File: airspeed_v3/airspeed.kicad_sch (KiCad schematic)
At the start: 27 parts, among them J1 Header, J2 GPS, J3 GPS, J4 ScreenIO, U1 XGZP6897D, U3 SHT4x, U5 XGZP6897D, U6 BME280, U8 BMP280

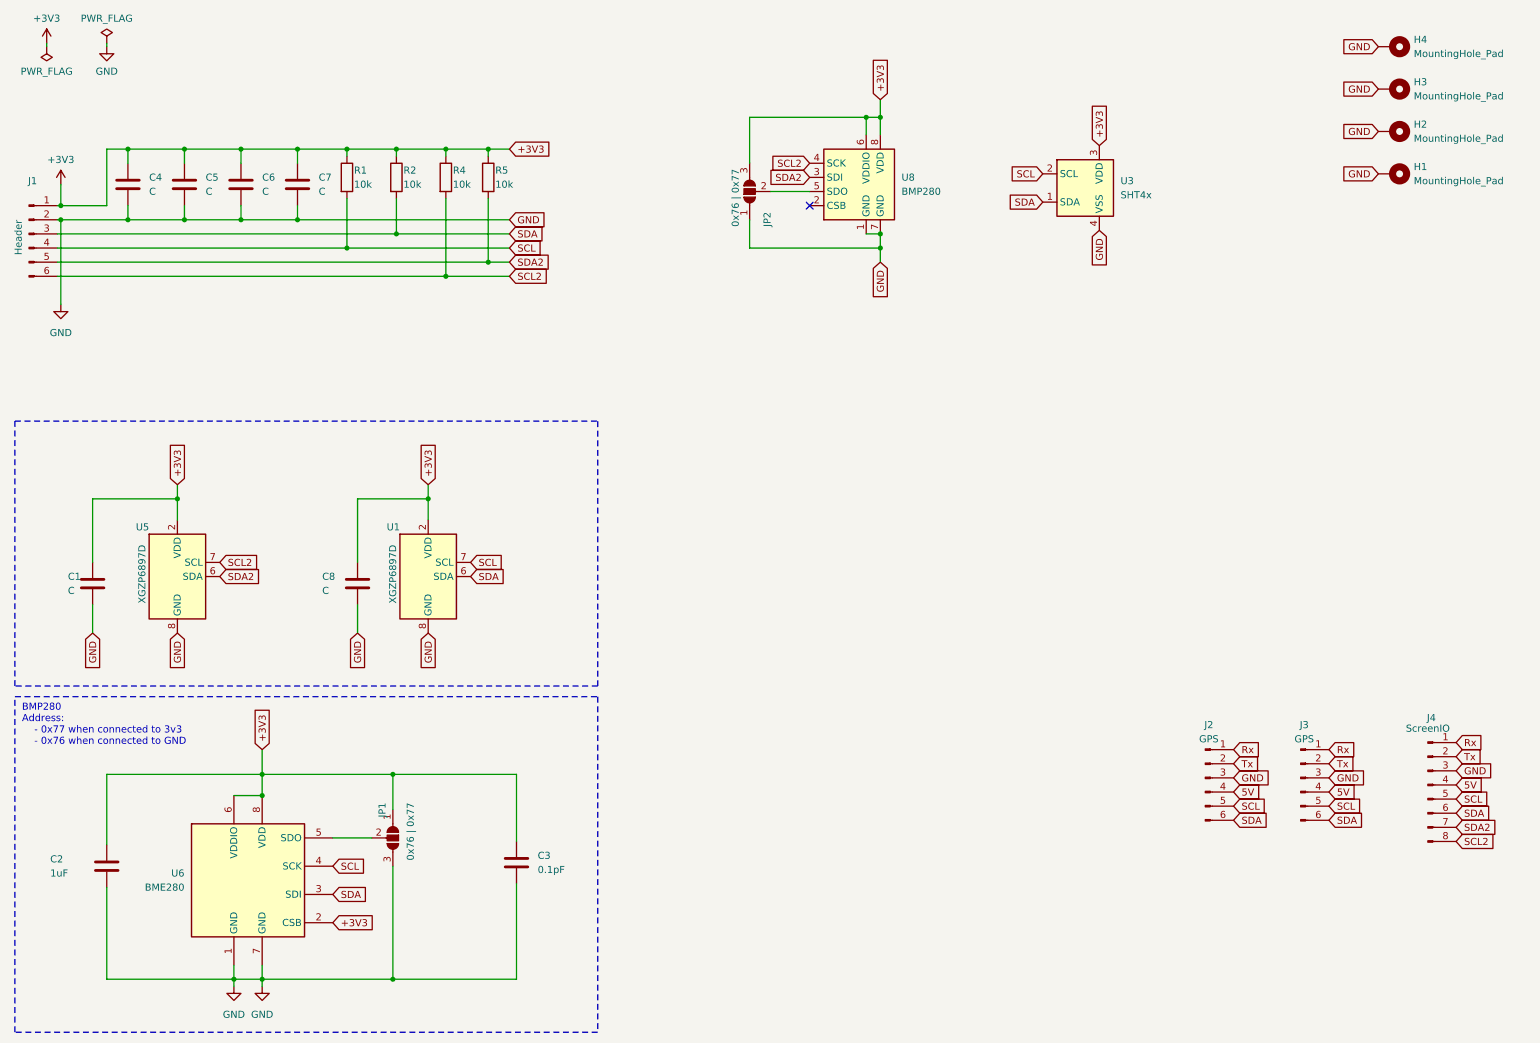
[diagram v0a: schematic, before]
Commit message: complete airspeed v3.2
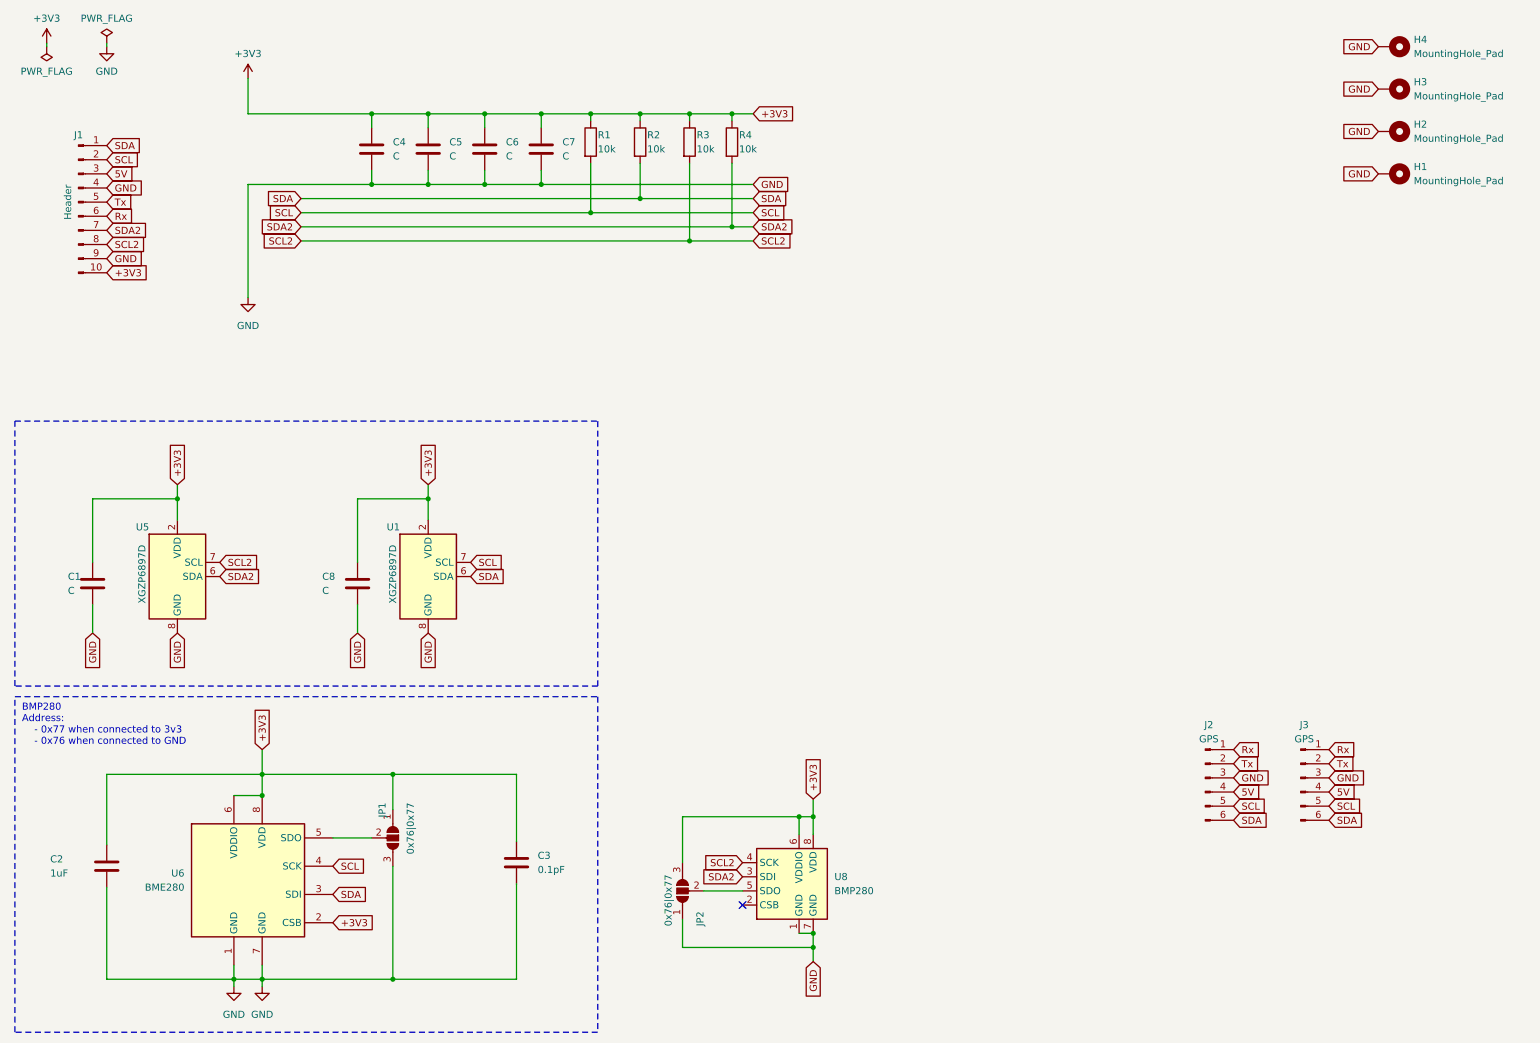
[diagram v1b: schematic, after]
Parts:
- removed J1: Header, Connector_PinHeader_2.54mm:PinHeader_1x06_P2.54mm_Vertical, symbol Connector:Conn_01x06_Pin
- removed J4: ScreenIO, Connector_PinHeader_1.27mm:PinHeader_1x08_P1.27mm_Vertical, symbol Connector:Conn_01x08_Pin
- removed R5: 10k, Resistor_SMD:R_0805_2012Metric, symbol Device:R
- removed U3: SHT4x, Sensor_Humidity:Sensirion_DFN-4_1.5x1.5mm_P0.8mm_SHT4x_NoCentralPad, symbol Sensor_Humidity:SHT4x
- added J1: Header, Connector_PinHeader_1.27mm:PinHeader_1x10_P1.27mm_Vertical, symbol Connector:Conn_01x10_Pin
- added R3: 10k, Resistor_SMD:R_0805_2012Metric, symbol Device:R
- JP1, JP2: value 0x76 | 0x77 -> 0x76|0x77; footprint Jumper:SolderJumper-3_P2.0mm_Open_TrianglePad1.0x1.5mm -> Jumper:SolderJumper-3_P1.3mm_Open_RoundedPad1.0x1.5mm
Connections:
- net +3V3: now also J1.10 (Pin_10), R3.1
- net 5V: now also J1.3 (Pin_3)
- net GND: now also J1.4 (Pin_4), J1.9 (Pin_9)
- net Rx: now also J1.6 (Pin_6)
- net SCL: now also J1.2 (Pin_2)
- net SCL2: now also J1.8 (Pin_8), R3.2; no longer R4.2
- net SDA: now also J1.1 (Pin_1)
- net SDA2: now also R4.2, J1.7 (Pin_7)
- net Tx: now also J1.5 (Pin_5)
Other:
- moved on the sheet: JP2, U8
